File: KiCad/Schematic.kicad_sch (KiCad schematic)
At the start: 44 parts, among them U4 LMH6609MF, U5 LMH6609MF, U6 LMH6609MF, U7 LMH6609MF, U8 LMH6609MF, U9 LMH6609MF

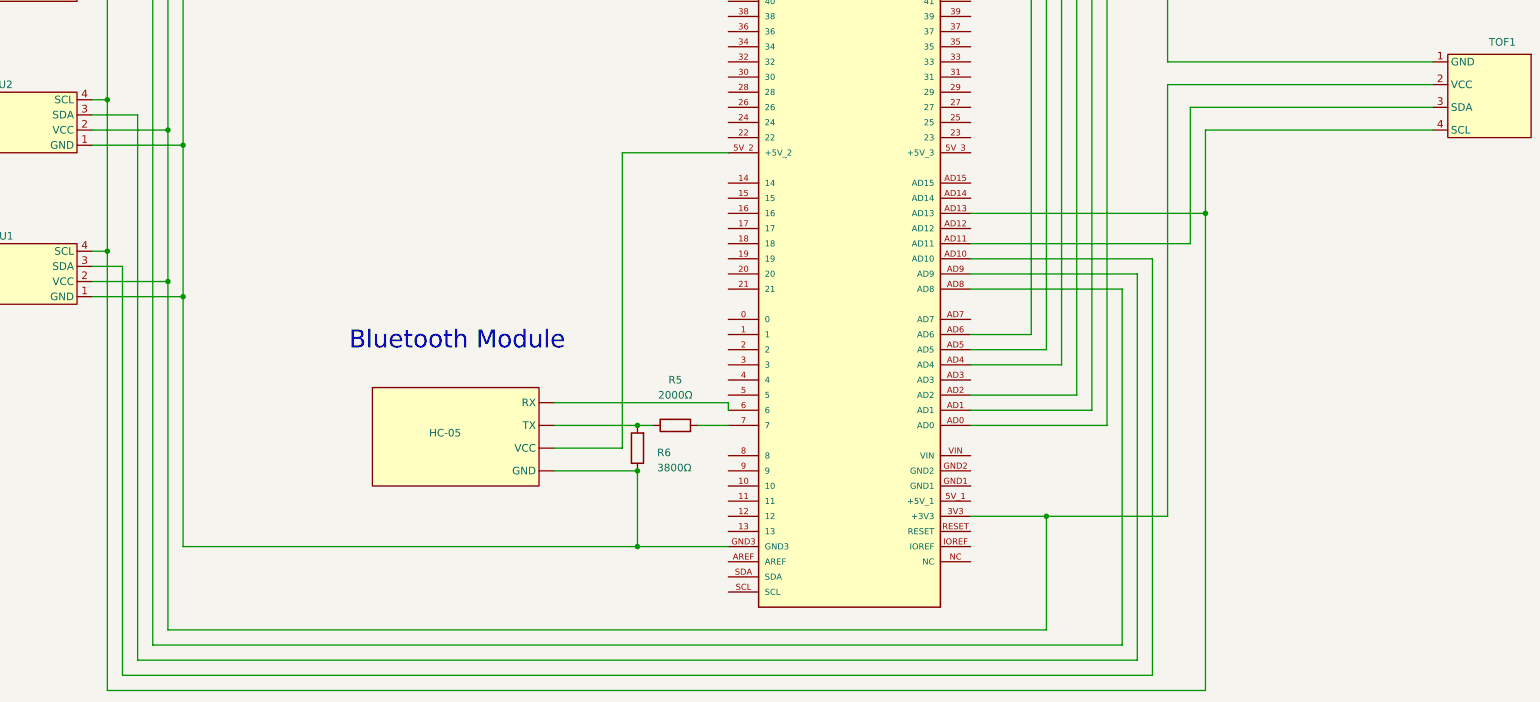
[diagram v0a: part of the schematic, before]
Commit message: Update Schematic.kicad_sch
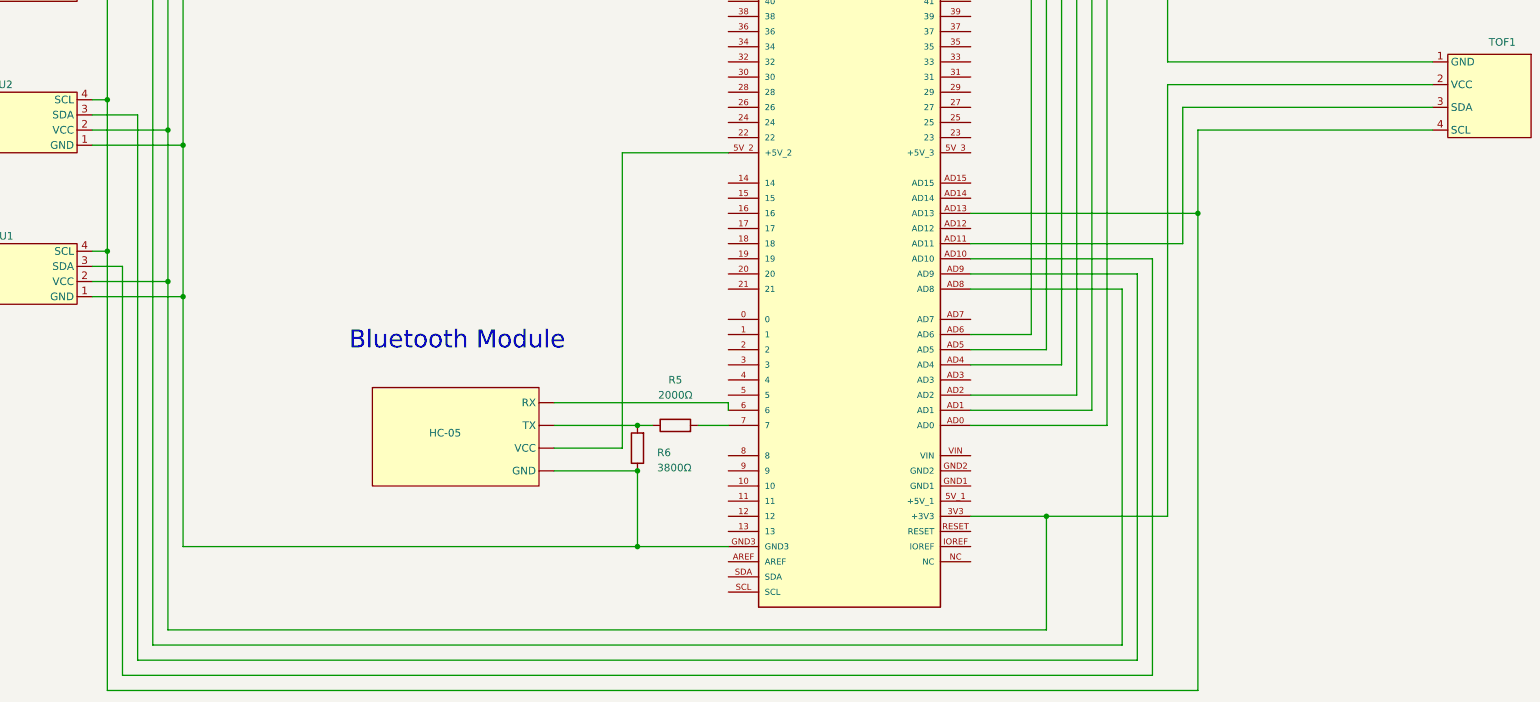
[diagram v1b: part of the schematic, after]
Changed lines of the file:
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@@
-	)
-	(junction
-		(at 280.67 190.5)
-		(diameter 0)
-		(color 0 0 0 0)
 	)
 	(junction
@@
 	)
 	(junction
+		(at 279.4 190.5)
+		(diameter 0)
+		(color 0 0 0 0)
+	)
+	(junction
 		(at 120.65 92.71)
 		(diameter 0)
@@
 	(wire
 		(pts
-			(xy 280.67 176.53) (xy 318.77 176.53)
+			(xy 279.4 176.53) (xy 318.77 176.53)
 		)
 		(stroke
@@
 	(wire
 		(pts
-			(xy 318.77 172.72) (xy 278.13 172.72)
-		)
-		(stroke
-			(width 0)
-			(type default)
-		)
-	)
-	(wire
-		(pts
-			(xy 96.52 270.51) (xy 280.67 270.51)
+			(xy 318.77 172.72) (xy 276.86 172.72)
+		)
+		(stroke
+			(width 0)
+			(type default)
+		)
+	)
+	(wire
+		(pts
+			(xy 96.52 270.51) (xy 279.4 270.51)
 		)
 		(stroke
@@
 	(wire
 		(pts
-			(xy 280.67 190.5) (xy 280.67 176.53)
+			(xy 279.4 190.5) (xy 279.4 176.53)
 		)
 		(stroke
@@
 	(wire
 		(pts
-			(xy 278.13 195.58) (xy 241.3 195.58)
+			(xy 276.86 195.58) (xy 241.3 195.58)
 		)
 		(stroke
@@
 	(wire
 		(pts
-			(xy 241.3 190.5) (xy 280.67 190.5)
+			(xy 241.3 190.5) (xy 279.4 190.5)
 		)
 		(stroke
@@
 	(wire
 		(pts
-			(xy 278.13 172.72) (xy 278.13 195.58)
-		)
-		(stroke
-			(width 0)
-			(type default)
-		)
-	)
-	(wire
-		(pts
-			(xy 280.67 270.51) (xy 280.67 190.5)
-		)
-		(stroke
+			(xy 276.86 172.72) (xy 276.86 195.58)
+		)
+		(stroke
+			(width 0)
+			(type default)
+		)
+	)
+	(wire
+		(pts
+			(xy 279.4 270.51) (xy 279.4 190.5)
+		)
+		(stroke
